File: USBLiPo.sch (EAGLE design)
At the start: 11 parts, among them IC1 LTC4054, J1 USB, J2 Li cell, Q1 2N7002

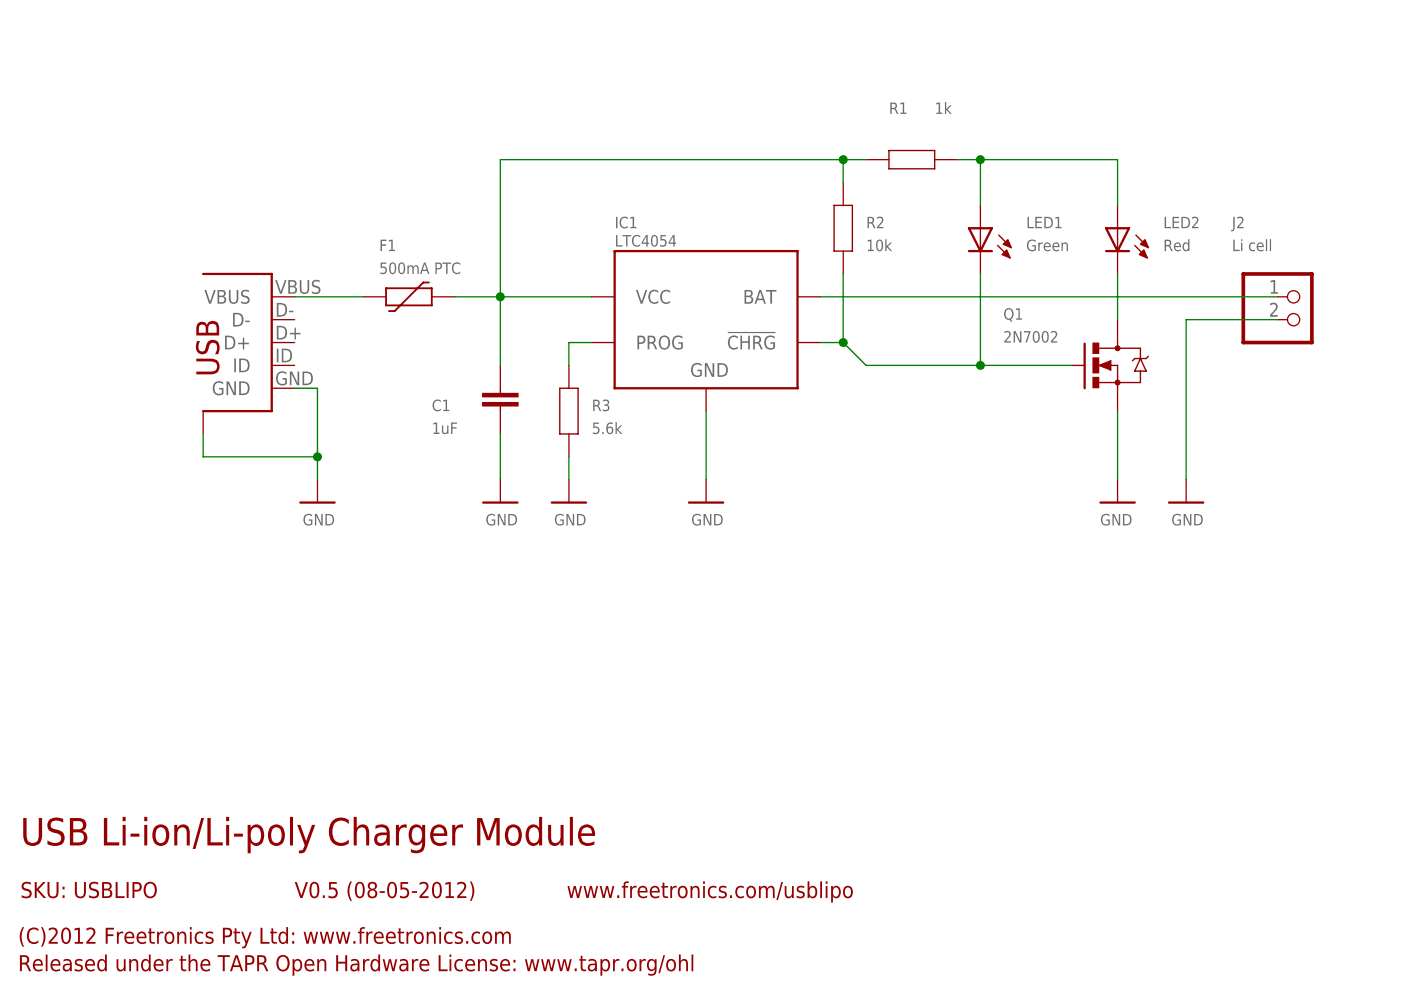
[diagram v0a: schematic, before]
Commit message: foo
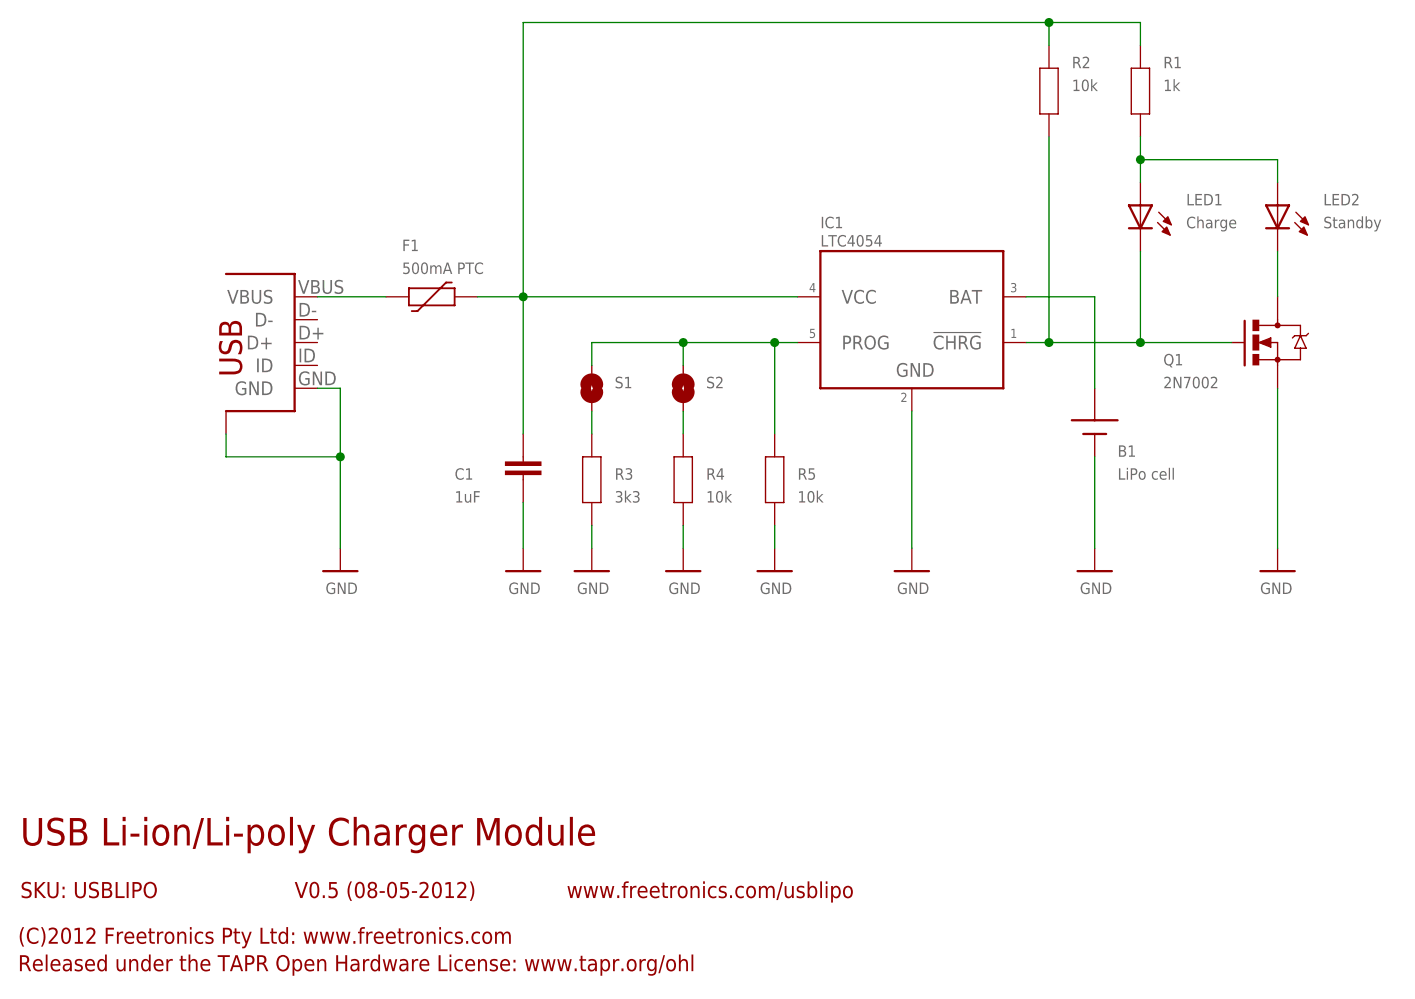
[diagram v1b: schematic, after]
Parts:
- removed J2: Li cell, adafruit:JST_2PIN-THM-RA
- added B1: LiPo cell, freetronics-luke:2P-JST-TH-RA
- added R4, R5: 10k, freetronics:RESISTOR0603
- added S1, S2: SJ, freetronics-luke:SJ
- LED1: value Green -> Charge
- LED2: value Red -> Standby
- R3: value 5.6k -> 3k3
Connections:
- new net N$5: R3.1, S1.1
- new net N$7: R4.1, S2.1
- net GND: now also B1.-, R4.2, R5.2; no longer J2.1
- net N$3: now also R5.1, S1.2, S2.2; no longer R3.1
- net N$4: now also B1.+; no longer J2.2
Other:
- note added: "0 0 100 mA"
- note added: "0 1 200 mA"
- note added: "1 0 403 mA"
- note added: "1 1 503 mA"
- note added: "2-pin 2.0mm JST"
- note added: "Green"
- note added: "S1 S2 Charge current"
- note added: "USER MUST ALWAYS DOUBLE CHECK BATTERY POLARITY BEFORE USE BECAUSE SOME LIPO CELLS ARE NOT STANDARD."
- note added: "Yellow"
- note removed: "2-pin SMD JST"
- note removed: "Iprog = 1000 V / 5600 ohms = 179 mA (Just a little under 0.2C for a typical 1.0 Ah LiPo cell.)"
- note removed: "JST CONNECTOR ORIENTATION/POLARITY MUST BE CHECKED. ARE ALL LIPO CELLS ``STANDARD''?"
- note removed: "Mates with LiPo cell."
- note removed: "Same as SparkFun one."
- note removed: "The FET allows two LEDs to be driven"
- note removed: "To do: Documentation of LED truth table, charging states."
- note removed: "USB shield connected to ground. Not completely sure if this is best."
- note removed: "from the LTC4054's open-drain output."
- moved on the sheet: C1, F1, LED1, LED2, Q1, R1, R2, R3
